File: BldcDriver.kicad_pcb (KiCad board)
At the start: 2 copper layers, 50 x 34 mm, 54 parts, among them J1 Motor Out, J2 DC Jack, J3 STM32_Debug_5pin, Q1 2SK4033, Q2 2SK4033, Q3 2SK4033, Q4 2SK4033, Q5 2SK4033, Q6 2SK4033, U1 IR2101, U2 IR2101, U3 IR2101, U4 NJM78L33SU3, U5 STM32F303K8Tx, X1 12MHz

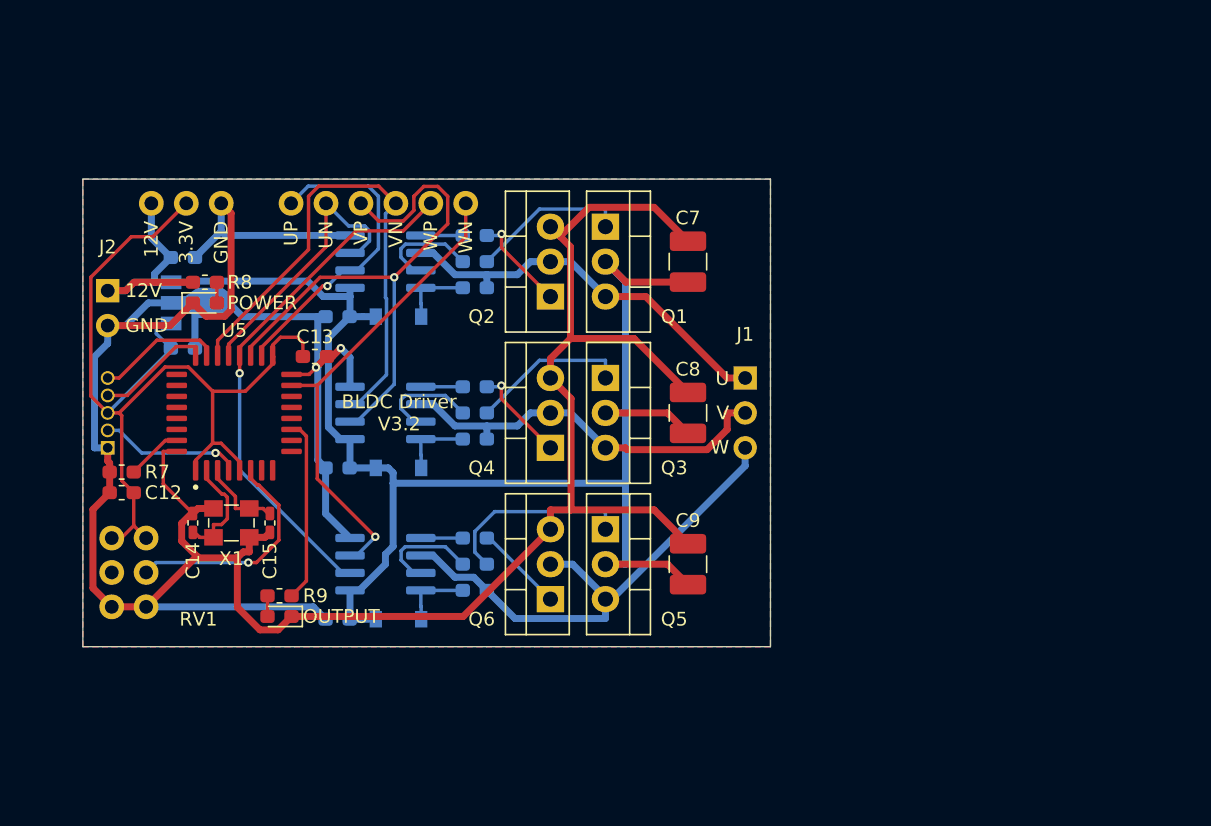
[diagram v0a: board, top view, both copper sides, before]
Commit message: 基板 V4.0
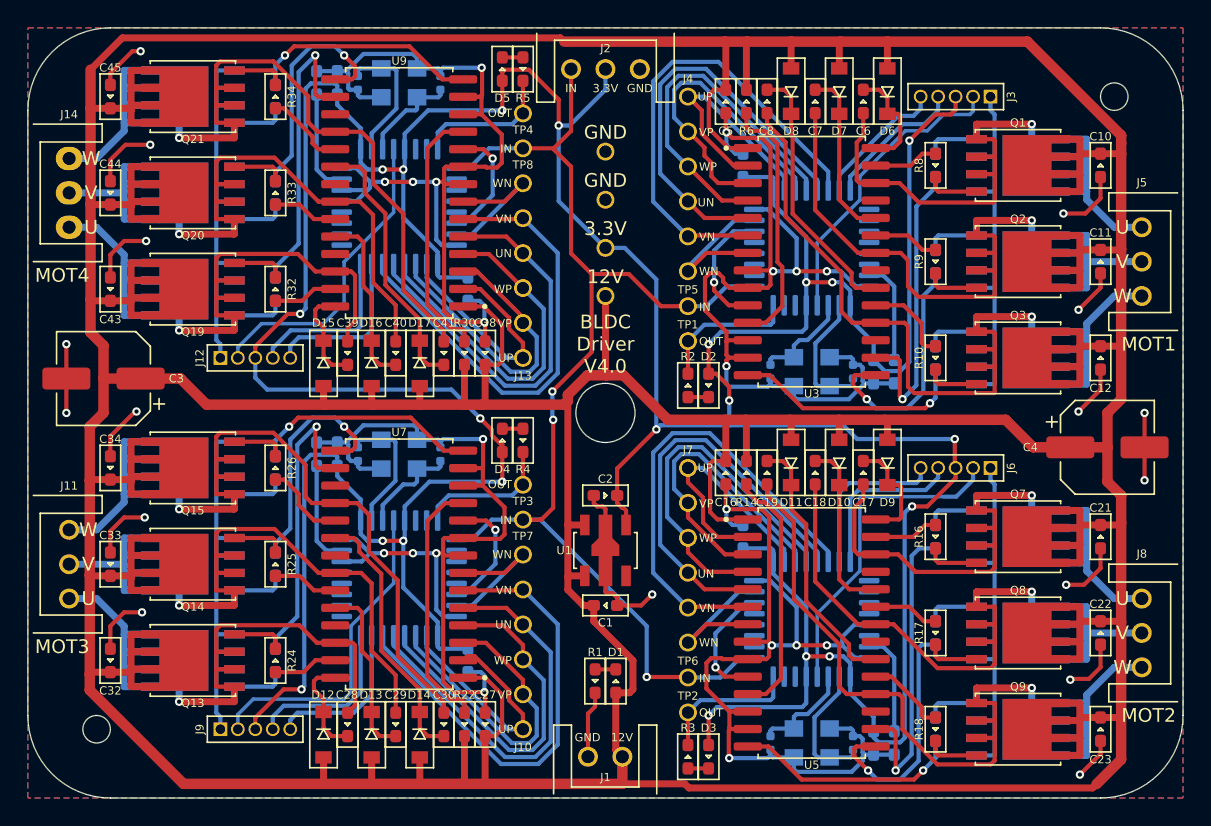
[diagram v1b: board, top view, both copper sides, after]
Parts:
- removed RV1: B10k, Potentiometer_THT:Potentiometer_Alps_RK097_Dual_Horizontal
- removed X1: 12MHz, BldcDriver:Crystal_SMD_3225-4Pin_3.2x2.5mm_HandSoldering
- added C16: 1uF, BldcDriver:1608Metric, F.Cu at (8.75, 4.35)
- added C17: 1uF, BldcDriver:1608Metric, F.Cu at (18.8, 4.35)
- added C18: 1uF, BldcDriver:1608Metric, F.Cu at (15.2, 4.35)
- added C19: 1uF, BldcDriver:1608Metric, F.Cu at (11.8, 4.35)
- added C20: 0.1uF, BldcDriver:1608Metric, B.Cu at (19.5, 24.0)
- added C21: 10uF, BldcDriver:1608Metric, F.Cu at (36.0, 9.00)
- added C22: 10uF, BldcDriver:1608Metric, F.Cu at (36.0, 16.0)
- added C23: 10uF, BldcDriver:1608Metric, F.Cu at (36.0, 23.0)
- added C24: 10pF, BldcDriver:1005Metric, B.Cu at (18.0, 24.0)
- added C25: 10pF, BldcDriver:1005Metric, B.Cu at (12.0, 24.0)
- added C26: 0.1uF, BldcDriver:1608Metric, B.Cu at (10.0, 9.00)
- added C27: 1uF, BldcDriver:1608Metric, F.Cu at (-8.75, 22.6)
- added C28: 1uF, BldcDriver:1608Metric, F.Cu at (-18.8, 22.6)
- added C29: 1uF, BldcDriver:1608Metric, F.Cu at (-15.2, 22.6)
- added C30: 1uF, BldcDriver:1608Metric, F.Cu at (-11.8, 22.6)
- added C31: 0.1uF, BldcDriver:1608Metric, B.Cu at (-19.5, 3.00)
- added C32: 10uF, BldcDriver:1608Metric, F.Cu at (-36.0, 18.0)
- added C33: 10uF, BldcDriver:1608Metric, F.Cu at (-36.0, 11.0)
- added C34: 10uF, BldcDriver:1608Metric, F.Cu at (-36.0, 4.00)
- added C35: 10pF, BldcDriver:1005Metric, B.Cu at (-18.0, 3.00)
- added C36: 10pF, BldcDriver:1005Metric, B.Cu at (-12.0, 3.00)
- added C37: 0.1uF, BldcDriver:1608Metric, B.Cu at (-10.0, 18.0)
- added C38: 1uF, BldcDriver:1608Metric, F.Cu at (-8.75, -4.35)
- added C39: 1uF, BldcDriver:1608Metric, F.Cu at (-18.8, -4.35)
- added C40: 1uF, BldcDriver:1608Metric, F.Cu at (-15.2, -4.35)
- added C41: 1uF, BldcDriver:1608Metric, F.Cu at (-11.8, -4.35)
- added C42: 0.1uF, BldcDriver:1608Metric, B.Cu at (-19.5, -24.0)
- added C43: 10uF, BldcDriver:1608Metric, F.Cu at (-36.0, -9.00)
- added C44: 10uF, BldcDriver:1608Metric, F.Cu at (-36.0, -16.0)
- added C45: 10uF, BldcDriver:1608Metric, F.Cu at (-36.0, -23.0)
- added C46: 10pF, BldcDriver:1005Metric, B.Cu at (-18.0, -24.0)
- added C47: 10pF, BldcDriver:1005Metric, B.Cu at (-12.0, -24.0)
- added C48: 0.1uF, BldcDriver:1608Metric, B.Cu at (-10.0, -9.00)
- added D10: 1N4148W, BldcDriver:D_SOD-123, F.Cu at (17.0, 3.60)
- added D11: 1N4148W, BldcDriver:D_SOD-123, F.Cu at (13.5, 3.60)
- added D12: 1N4148W, BldcDriver:D_SOD-123, F.Cu at (-20.5, 23.4)
- added D13: 1N4148W, BldcDriver:D_SOD-123, F.Cu at (-17.0, 23.4)
- added D14: 1N4148W, BldcDriver:D_SOD-123, F.Cu at (-13.5, 23.4)
- added D15: 1N4148W, BldcDriver:D_SOD-123, F.Cu at (-20.5, -3.60)
- added D16: 1N4148W, BldcDriver:D_SOD-123, F.Cu at (-17.0, -3.60)
- added D17: 1N4148W, BldcDriver:D_SOD-123, F.Cu at (-13.5, -3.60)
- added D6: 1N4148W, BldcDriver:D_SOD-123, F.Cu at (20.5, -23.4)
- added D7: 1N4148W, BldcDriver:D_SOD-123, F.Cu at (17.0, -23.4)
- added D8: 1N4148W, BldcDriver:D_SOD-123, F.Cu at (13.5, -23.4)
- added D9: 1N4148W, BldcDriver:D_SOD-123, F.Cu at (20.5, 3.60)
- added H1: MountingHole, BldcDriver:MountingHole_4.3mm_M4, F.Cu at (0.00, 0.00)
- added H2: MountingHole, BldcDriver:MountingHole_2mm, F.Cu at (37.0, -23.0)
- added H3: MountingHole, BldcDriver:MountingHole_2mm, F.Cu at (-37.0, 23.0)
- added J10: Conn_01x06, BldcDriver:Pin_1x06_P2.54mm, F.Cu at (-6.00, 23.0)
- added J11: MOTOR_OUT, BldcDriver:JST_XH_S3B-XH-A_1x03_P2.50mm_Horizontal, F.Cu at (-39.0, 8.50)
- added J12: STM32_Debug, BldcDriver:STM32_Debug_5pin, F.Cu at (-28.0, -4.00)
- added J13: Conn_01x06, BldcDriver:Pin_1x06_P2.54mm, F.Cu at (-6.00, -4.00)
- added J14: MOTOR_OUT, BldcDriver:JST_XH_S3B-XH-A_1x03_P2.50mm_Horizontal, F.Cu at (-39.0, -18.5)
- added J4: Conn_01x06, BldcDriver:Pin_1x06_P2.54mm, F.Cu at (6.00, -23.0)
- added J5: MOTOR_OUT, BldcDriver:JST_XH_S3B-XH-A_1x03_P2.50mm_Horizontal, F.Cu at (39.0, -8.50)
- added J6: STM32_Debug, BldcDriver:STM32_Debug_5pin, F.Cu at (28.0, 4.00)
- added J7: Conn_01x06, BldcDriver:Pin_1x06_P2.54mm, F.Cu at (6.00, 4.00)
- added J8: MOTOR_OUT, BldcDriver:JST_XH_S3B-XH-A_1x03_P2.50mm_Horizontal, F.Cu at (39.0, 18.5)
- added J9: STM32_Debug, BldcDriver:STM32_Debug_5pin, F.Cu at (-28.0, 23.0)
- added Q10: IRFH7545, BldcDriver:VSONP-8-1EP_5x6_P1.27mm, B.Cu at (30.0, 9.00)
- added Q11: IRFH7545, BldcDriver:VSONP-8-1EP_5x6_P1.27mm, B.Cu at (30.0, 16.0)
- added Q12: IRFH7545, BldcDriver:VSONP-8-1EP_5x6_P1.27mm, B.Cu at (30.0, 23.0)
- added Q13: IRFH7545, BldcDriver:VSONP-8-1EP_5x6_P1.27mm, F.Cu at (-30.0, 18.0)
- added Q14: IRFH7545, BldcDriver:VSONP-8-1EP_5x6_P1.27mm, F.Cu at (-30.0, 11.0)
- added Q15: IRFH7545, BldcDriver:VSONP-8-1EP_5x6_P1.27mm, F.Cu at (-30.0, 4.00)
- added Q16: IRFH7545, BldcDriver:VSONP-8-1EP_5x6_P1.27mm, B.Cu at (-30.0, 18.0)
- added Q17: IRFH7545, BldcDriver:VSONP-8-1EP_5x6_P1.27mm, B.Cu at (-30.0, 11.0)
- added Q18: IRFH7545, BldcDriver:VSONP-8-1EP_5x6_P1.27mm, B.Cu at (-30.0, 4.00)
- added Q19: IRFH7545, BldcDriver:VSONP-8-1EP_5x6_P1.27mm, F.Cu at (-30.0, -9.00)
- added Q20: IRFH7545, BldcDriver:VSONP-8-1EP_5x6_P1.27mm, F.Cu at (-30.0, -16.0)
- added Q21: IRFH7545, BldcDriver:VSONP-8-1EP_5x6_P1.27mm, F.Cu at (-30.0, -23.0)
- added Q22: IRFH7545, BldcDriver:VSONP-8-1EP_5x6_P1.27mm, B.Cu at (-30.0, -9.00)
- added Q23: IRFH7545, BldcDriver:VSONP-8-1EP_5x6_P1.27mm, B.Cu at (-30.0, -16.0)
- added Q24: IRFH7545, BldcDriver:VSONP-8-1EP_5x6_P1.27mm, B.Cu at (-30.0, -23.0)
- added Q7: IRFH7545, BldcDriver:VSONP-8-1EP_5x6_P1.27mm, F.Cu at (30.0, 9.00)
- added Q8: IRFH7545, BldcDriver:VSONP-8-1EP_5x6_P1.27mm, F.Cu at (30.0, 16.0)
- added Q9: IRFH7545, BldcDriver:VSONP-8-1EP_5x6_P1.27mm, F.Cu at (30.0, 23.0)
- added R10: 100, BldcDriver:1608Metric, F.Cu at (24.0, -4.00)
- added R11: 100, BldcDriver:1608Metric, B.Cu at (24.0, -18.0)
- added R12: 100, BldcDriver:1608Metric, B.Cu at (24.0, -11.0)
- added R13: 100, BldcDriver:1608Metric, B.Cu at (24.0, -4.00)
- added R14: 10k, BldcDriver:1608Metric, F.Cu at (10.2, 4.35)
- added R15: 10k, BldcDriver:1608Metric, B.Cu at (21.0, 24.0)
- added R16: 100, BldcDriver:1608Metric, F.Cu at (24.0, 9.00)
- added R17: 100, BldcDriver:1608Metric, F.Cu at (24.0, 16.0)
- added R18: 100, BldcDriver:1608Metric, F.Cu at (24.0, 23.0)
- added R19: 100, BldcDriver:1608Metric, B.Cu at (24.0, 9.00)
- added R20: 100, BldcDriver:1608Metric, B.Cu at (24.0, 16.0)
- added R21: 100, BldcDriver:1608Metric, B.Cu at (24.0, 23.0)
- added R22: 10k, BldcDriver:1608Metric, F.Cu at (-10.2, 22.6)
- added R23: 10k, BldcDriver:1608Metric, B.Cu at (-21.0, 3.00)
- added R24: 100, BldcDriver:1608Metric, F.Cu at (-24.0, 18.0)
- added R25: 100, BldcDriver:1608Metric, F.Cu at (-24.0, 11.0)
- added R26: 100, BldcDriver:1608Metric, F.Cu at (-24.0, 4.00)
- added R27: 100, BldcDriver:1608Metric, B.Cu at (-24.0, 18.0)
- added R28: 100, BldcDriver:1608Metric, B.Cu at (-24.0, 11.0)
- added R29: 100, BldcDriver:1608Metric, B.Cu at (-24.0, 4.00)
- added R30: 10k, BldcDriver:1608Metric, F.Cu at (-10.2, -4.35)
- added R31: 10k, BldcDriver:1608Metric, B.Cu at (-21.0, -24.0)
- added R32: 100, BldcDriver:1608Metric, F.Cu at (-24.0, -9.00)
- added R33: 100, BldcDriver:1608Metric, F.Cu at (-24.0, -16.0)
- added R34: 100, BldcDriver:1608Metric, F.Cu at (-24.0, -23.0)
- added R35: 100, BldcDriver:1608Metric, B.Cu at (-24.0, -9.00)
- added R36: 100, BldcDriver:1608Metric, B.Cu at (-24.0, -16.0)
- added R37: 100, BldcDriver:1608Metric, B.Cu at (-24.0, -23.0)
- added TP10: TestPoint, BldcDriver:TestPoint_THTPad_D1.3mm_Drill0.9mm, F.Cu at (0.00, -12.0)
- added TP11: TestPoint, BldcDriver:TestPoint_THTPad_D1.3mm_Drill0.9mm, F.Cu at (0.00, -15.5)
- added TP12: TestPoint, BldcDriver:TestPoint_THTPad_D1.3mm_Drill0.9mm, F.Cu at (0.00, -19.0)
- added U6: STM32F303K8Tx, BldcDriver:LQFP-32_7x7mm_P0.8mm_FusionPCB, B.Cu at (-15.0, 12.0)
- added U7: IR2136S, BldcDriver:SOIC-28W_7.5x17.9mm_P1.27mm, F.Cu at (-15.0, 11.0)
- added U8: STM32F303K8Tx, BldcDriver:LQFP-32_7x7mm_P0.8mm_FusionPCB, B.Cu at (-15.0, -15.0)
- added U9: IR2136S, BldcDriver:SOIC-28W_7.5x17.9mm_P1.27mm, F.Cu at (-15.0, -16.0)
- added Y1: 12MHz, BldcDriver:Crystal_SMD_3225-4Pin_3.2x2.5mm_HandSoldering, B.Cu at (15.0, -3.00)
- added Y2: 12MHz, BldcDriver:Crystal_SMD_3225-4Pin_3.2x2.5mm_HandSoldering, B.Cu at (15.0, 24.0)
- added Y3: 12MHz, BldcDriver:Crystal_SMD_3225-4Pin_3.2x2.5mm_HandSoldering, B.Cu at (-15.0, 3.00)
- added Y4: 12MHz, BldcDriver:Crystal_SMD_3225-4Pin_3.2x2.5mm_HandSoldering, B.Cu at (-15.0, -24.0)
- C1: value 10uF -> 0.33uF; footprint Capacitor_SMD:C_0603_1608Metric_Pad1.05x0.95mm_HandSolder -> BldcDriver:1608Metric; moved to F.Cu
- C10: value 0.39uF -> 10uF; footprint Capacitor_SMD:C_0603_1608Metric_Pad1.05x0.95mm_HandSolder -> BldcDriver:1608Metric; moved to F.Cu
- C11: value 0.1uF -> 10uF; footprint Capacitor_SMD:C_0603_1608Metric_Pad1.05x0.95mm_HandSolder -> BldcDriver:1608Metric; moved to F.Cu
- C12: value 0.1uF -> 10uF; footprint Capacitor_SMD:C_0603_1608Metric_Pad1.05x0.95mm_HandSolder -> BldcDriver:1608Metric
- C13: value 0.1uF -> 10pF; footprint Capacitor_SMD:C_0603_1608Metric_Pad1.05x0.95mm_HandSolder -> BldcDriver:1005Metric; moved to B.Cu
- C14: footprint BldcDriver:C_0402_1005Metric -> BldcDriver:1005Metric; moved to B.Cu
- C15: value 10pF -> 0.1uF; footprint BldcDriver:C_0402_1005Metric -> BldcDriver:1608Metric; moved to B.Cu
- C2: value 10uF -> 2.2uF; footprint Capacitor_SMD:C_0603_1608Metric_Pad1.05x0.95mm_HandSolder -> BldcDriver:1608Metric; moved to F.Cu
- C3, C4: value 10uF -> 100uF; footprint Capacitor_SMD:C_0603_1608Metric_Pad1.05x0.95mm_HandSolder -> BldcDriver:CP_Elec_6.3x7.7; moved to F.Cu
- C5, C6: value 10uF -> 1uF; footprint Capacitor_SMD:C_0603_1608Metric_Pad1.05x0.95mm_HandSolder -> BldcDriver:1608Metric; moved to F.Cu
- C7, C8: value 22uF -> 1uF; footprint Capacitor_SMD:C_1210_3225Metric_Pad1.42x2.65mm_HandSolder -> BldcDriver:1608Metric
- C9: value 22uF -> 0.1uF; footprint Capacitor_SMD:C_1210_3225Metric_Pad1.42x2.65mm_HandSolder -> BldcDriver:1608Metric; moved to B.Cu
- D1: value 1N4148W -> Power; footprint Diode_SMD:D_SOD-123 -> BldcDriver:1608Metric; moved to F.Cu
- D2: value 1N4148W -> OUT1; footprint Diode_SMD:D_SOD-123 -> BldcDriver:1608Metric; moved to F.Cu
- D3: value 1N4148W -> OUT2; footprint Diode_SMD:D_SOD-123 -> BldcDriver:1608Metric; moved to F.Cu
- D4: value Power -> OUT3; footprint LED_SMD:LED_0603_1608Metric_Pad1.05x0.95mm_HandSolder -> BldcDriver:1608Metric
- D5: value Output -> OUT4; footprint LED_SMD:LED_0603_1608Metric_Pad1.05x0.95mm_HandSolder -> BldcDriver:1608Metric
- J1: value Motor Out -> POWER; footprint Connector_PinSocket_2.54mm:PinSocket_1x03_P2.54mm_Vertical -> BldcDriver:JST_XH_S2B-XH-A_1x02_P2.50mm_Horizontal
- J2: value DC Jack -> CONTROL; footprint Connector_PinSocket_2.54mm:PinSocket_1x02_P2.54mm_Vertical -> BldcDriver:JST_XH_S3B-XH-A_1x03_P2.50mm_Horizontal
- J3: value STM32_Debug_5pin -> STM32_Debug; moved to F.Cu
- Q1, Q2, Q3: value 2SK4033 -> IRFH7545; footprint Package_TO_SOT_THT:TO-220-3_Vertical -> BldcDriver:VSONP-8-1EP_5x6_P1.27mm
- Q4, Q5, Q6: value 2SK4033 -> IRFH7545; footprint Package_TO_SOT_THT:TO-220-3_Vertical -> BldcDriver:VSONP-8-1EP_5x6_P1.27mm; moved to B.Cu
- R1, R2, R3, R4, R5: value 100 -> R; footprint Resistor_SMD:R_0603_1608Metric_Pad1.05x0.95mm_HandSolder -> BldcDriver:1608Metric; moved to F.Cu
- R6: value 100 -> 10k; footprint Resistor_SMD:R_0603_1608Metric_Pad1.05x0.95mm_HandSolder -> BldcDriver:1608Metric; moved to F.Cu
- R7: footprint Resistor_SMD:R_0603_1608Metric_Pad1.05x0.95mm_HandSolder -> BldcDriver:1608Metric; moved to B.Cu
- R8, R9: value R -> 100; footprint Resistor_SMD:R_0603_1608Metric_Pad1.05x0.95mm_HandSolder -> BldcDriver:1608Metric
- TP1: value +12V -> TestPoint; footprint BldcDriver:TestPoint_THTPad_D2.0mm_Drill1.0mm -> BldcDriver:TestPoint_THTPad_D1.3mm_Drill0.9mm
- TP2: value GND -> TestPoint; footprint BldcDriver:TestPoint_THTPad_D2.0mm_Drill1.0mm -> BldcDriver:TestPoint_THTPad_D1.3mm_Drill0.9mm
- TP3: value 3.3V -> TestPoint; footprint BldcDriver:TestPoint_THTPad_D2.0mm_Drill1.0mm -> BldcDriver:TestPoint_THTPad_D1.3mm_Drill0.9mm
- TP4: value UP -> TestPoint; footprint BldcDriver:TestPoint_THTPad_D2.0mm_Drill1.0mm -> BldcDriver:TestPoint_THTPad_D1.3mm_Drill0.9mm
- TP5: value UN -> TestPoint; footprint BldcDriver:TestPoint_THTPad_D2.0mm_Drill1.0mm -> BldcDriver:TestPoint_THTPad_D1.3mm_Drill0.9mm
- TP6: value VP -> TestPoint; footprint BldcDriver:TestPoint_THTPad_D2.0mm_Drill1.0mm -> BldcDriver:TestPoint_THTPad_D1.3mm_Drill0.9mm
- TP7: value VN -> TestPoint; footprint BldcDriver:TestPoint_THTPad_D2.0mm_Drill1.0mm -> BldcDriver:TestPoint_THTPad_D1.3mm_Drill0.9mm
- TP8: value WP -> TestPoint; footprint BldcDriver:TestPoint_THTPad_D2.0mm_Drill1.0mm -> BldcDriver:TestPoint_THTPad_D1.3mm_Drill0.9mm
- TP9: value WN -> TestPoint; footprint BldcDriver:TestPoint_THTPad_D2.0mm_Drill1.0mm -> BldcDriver:TestPoint_THTPad_D1.3mm_Drill0.9mm
- U1: value IR2101 -> NJM2884U1; footprint BldcDriver:SOIC-8_3.9x4.9mm_P1.27mm -> BldcDriver:SOT-89-5; moved to F.Cu
- U2: value IR2101 -> STM32F303K8Tx; footprint BldcDriver:SOIC-8_3.9x4.9mm_P1.27mm -> BldcDriver:LQFP-32_7x7mm_P0.8mm_FusionPCB
- U3: value IR2101 -> IR2136S; footprint BldcDriver:SOIC-8_3.9x4.9mm_P1.27mm -> BldcDriver:SOIC-28W_7.5x17.9mm_P1.27mm; moved to F.Cu
- U4: value NJM78L33SU3 -> STM32F303K8Tx; footprint Package_TO_SOT_SMD:SOT-89-3 -> BldcDriver:LQFP-32_7x7mm_P0.8mm_FusionPCB
- U5: value STM32F303K8Tx -> IR2136S; footprint BldcDriver:LQFP-32_7x7mm_P0.8mm_FusionPCB -> BldcDriver:SOIC-28W_7.5x17.9mm_P1.27mm
- moved C12 71.8 mm to (36.0, -4.00), turned to 270 degrees
- moved J3 69.1 mm to (28.0, -23.0), turned to 270 degrees
- moved C10 67.1 mm to (36.0, -18.0), turned to 270 degrees
- moved C11 67.0 mm to (36.0, -11.0), turned to 270 degrees
- moved R7 56.6 mm to (21.0, -3.00), turned to 270 degrees
- moved R8 53.8 mm to (24.0, -18.0), turned to 90 degrees
- moved R9 53.5 mm to (24.0, -11.0), turned to 90 degrees
- moved U4 50.6 mm to (15.0, 15.0), turned to 90 degrees
- moved TP2 50.2 mm to (6.00, 21.8)
- moved C4 47.4 mm to (36.5, 2.50)
- moved C6 45.4 mm to (18.8, -22.6), turned to 270 degrees
- moved C15 45.3 mm to (19.5, -3.00)
- moved U5 44.9 mm to (15.0, 16.0), turned to 0 degrees
- moved C14 43.4 mm to (12.0, -3.00), turned to 270 degrees
- moved D5 43.0 mm to (-7.50, -25.0), turned to 270 degrees
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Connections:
- C11 pad 1: +3V3 -> +12V
- C12 pad 1: +3V3 -> +12V
- C13 pad 1: +3V3 -> GND
- C13 pad 2: GND -> Net-(C13-Pad2)
- C14 pad 1: OSC_I -> Net-(C14-Pad1)
- C15 pad 1: OSC_O -> +3V3
- C2 pad 1: +12V -> +3V3
- C4 pad 1: Net-(C4-Pad1) -> +12V
- C4 pad 2: /U -> GND
- C5 pad 1: Net-(C5-Pad1) -> +12V
- C5 pad 2: /V -> GND
- C6 pad 2: /W -> /U1
- C7 pad 1: +12V -> Net-(C7-Pad1)
- C7 pad 2: GND -> /V1
- C8 pad 1: +12V -> Net-(C8-Pad1)
- C8 pad 2: GND -> /W1
- C9 pad 1: +12V -> +3V3
- D1 pad 1: Net-(C4-Pad1) -> Net-(D1-Pad1)
- D2 pad 1: Net-(C5-Pad1) -> Net-(D2-Pad1)
- D2 pad 2: +12V -> +3V3
- D3 pad 1: Net-(C6-Pad1) -> Net-(D3-Pad1)
- D3 pad 2: +12V -> +3V3
- D4 pad 1: GND -> Net-(D4-Pad1)
- D4 pad 2: Net-(D4-Pad2) -> +3V3
- D5 pad 1: GND -> Net-(D5-Pad1)
- D5 pad 2: Net-(D5-Pad2) -> +3V3
- J1 pad 1: /U -> +12V
- J1 pad 2: /V -> GND
- J2 pad 1: +12V -> IN1
- J2 pad 2: GND -> +3V3
- J3 pad 2: NRST -> Net-(J3-Pad2)
- J3 pad 4: SWCLK -> Net-(J3-Pad4)
- J3 pad 5: SWDIO -> Net-(J3-Pad5)
- Q1 pad 1: Net-(Q1-Pad1) -> /U1
- Q1 pad 2: +12V -> Net-(Q1-Pad2)
- Q1 pad 3: /U -> +12V
- Q2 pad 1: Net-(Q2-Pad1) -> /V1
- Q2 pad 2: /U -> Net-(Q2-Pad2)
- Q2 pad 3: GND -> +12V
- Q3 pad 1: Net-(Q3-Pad1) -> /W1
- Q3 pad 2: +12V -> Net-(Q3-Pad2)
- Q3 pad 3: /V -> +12V
- Q4 pad 1: Net-(Q4-Pad1) -> GND
- Q4 pad 2: /V -> Net-(Q4-Pad2)
- Q4 pad 3: GND -> /U1
- Q5 pad 1: Net-(Q5-Pad1) -> GND
- Q5 pad 2: +12V -> Net-(Q5-Pad2)
- Q5 pad 3: /W -> /V1
- Q6 pad 1: Net-(Q6-Pad1) -> GND
- Q6 pad 2: /W -> Net-(Q6-Pad2)
- Q6 pad 3: GND -> /W1
- R1 pad 1: Net-(Q1-Pad1) -> GND
- R1 pad 2: Net-(R1-Pad2) -> Net-(D1-Pad1)
- R2 pad 1: Net-(Q2-Pad1) -> OUT1
- R2 pad 2: Net-(R2-Pad2) -> Net-(D2-Pad1)
- R3 pad 1: Net-(Q3-Pad1) -> OUT2
- R3 pad 2: Net-(R3-Pad2) -> Net-(D3-Pad1)
- R4 pad 1: Net-(Q4-Pad1) -> OUT3
- R4 pad 2: Net-(R4-Pad2) -> Net-(D4-Pad1)
- R5 pad 1: Net-(Q5-Pad1) -> OUT4
- R5 pad 2: Net-(R5-Pad2) -> Net-(D5-Pad1)
- R6 pad 1: Net-(Q6-Pad1) -> +12V
- R8 pad 1: Net-(D4-Pad2) -> Net-(Q1-Pad2)
- R8 pad 2: +12V -> Net-(R8-Pad2)
- R9 pad 1: Net-(D5-Pad2) -> Net-(Q2-Pad2)
- R9 pad 2: LED -> Net-(R9-Pad2)
- TP1 pad 1: +12V -> OUT1
- TP2 pad 1: GND -> OUT2
- TP3 pad 1: +3V3 -> OUT3
- TP4 pad 1: UP -> OUT4
- TP5 pad 1: UN -> IN1
- TP6 pad 1: VP -> IN1
- TP7 pad 1: VN -> IN1
- TP8 pad 1: WP -> IN1
- TP9 pad 1: WN -> +12V
- U1 pad 2: UP -> GND
- U1 pad 3: UN -> Net-(U1-Pad3)
- U1 pad 4: GND -> +3V3
- U1 pad 5: Net-(R2-Pad2) -> +12V
- U2 pad 1: +12V -> +3V3
- U2 pad 2: VP -> Net-(C13-Pad2)
- U2 pad 3: VN -> Net-(C14-Pad1)
- U2 pad 4: GND -> Net-(J3-Pad2)
- U2 pad 5: Net-(R4-Pad2) -> +3V3
- U2 pad 6: /V -> Net-(U2-Pad6)
- U2 pad 7: Net-(R3-Pad2) -> Net-(U2-Pad7)
- U2 pad 8: Net-(C5-Pad1) -> OUT1
- U3 pad 2: WP -> /UP1
- U3 pad 3: WN -> /VP1
- U3 pad 4: GND -> /WP1
- U3 pad 5: Net-(R6-Pad2) -> /UN1
- U3 pad 6: /W -> /VN1
- U3 pad 7: Net-(R5-Pad2) -> /WN1
- U3 pad 8: Net-(C6-Pad1) -> GND
- U4 pad 2: GND -> Net-(C24-Pad2)
- U4 pad 3: +12V -> Net-(C25-Pad1)
- U5 pad 1: +3V3 -> +12V
- U5 pad 10: (no net) -> Net-(U4-Pad14)
- U5 pad 11: LED -> Net-(R14-Pad2)
- U5 pad 12: (no net) -> GND
- U5 pad 13: (no net) -> GND
- U5 pad 14: (no net) -> Net-(R21-Pad2)
- U5 pad 15: WN -> Net-(R20-Pad2)
- U5 pad 16: GND -> Net-(R19-Pad2)
- U5 pad 17: +3V3 -> Net-(U5-Pad17)
- U5 pad 18: UP -> /W2
- U5 pad 19: VP -> Net-(R18-Pad2)
- U5 pad 2: OSC_I -> /UP2
- U5 pad 20: WP -> Net-(C19-Pad1)
- U5 pad 21: UN -> Net-(U5-Pad21)
- U5 pad 22: VN -> /V2
- U5 pad 23: SWDIO -> Net-(R17-Pad2)
- U5 pad 24: SWCLK -> Net-(C18-Pad1)
- U5 pad 25: (no net) -> Net-(U5-Pad25)
- U5 pad 26: (no net) -> /U2
- U5 pad 27: (no net) -> Net-(R16-Pad2)
- U5 pad 28: (no net) -> Net-(C17-Pad1)
- U5 pad 3: OSC_O -> /VP2
- U5 pad 4: NRST -> /WP2
- U5 pad 5: +3V3 -> /UN2
- U5 pad 6: ADC -> /VN2
- U5 pad 7: (no net) -> /WN2
- U5 pad 8: (no net) -> GND
- U5 pad 9: (no net) -> GND
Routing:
- net +12V: track 128.1 -> 625.7 mm
- net +3V3: track 70.7 -> 329.5 mm, vias 0 -> 21
- net GND: track 226.5 -> 484.3 mm, vias 2 -> 37
- net IN1: track 0.00 -> 88.1 mm, vias 0 -> 3
- net /W1: track 0.00 -> 69.0 mm, vias 0 -> 1
- net /W2: track 0.00 -> 68.0 mm, vias 0 -> 1
- net /W3: track 0.00 -> 67.7 mm, vias 0 -> 1
- net /W4: track 0.00 -> 67.7 mm, vias 0 -> 1
- net /V1: track 0.00 -> 58.6 mm, vias 0 -> 1
- net /V3: track 0.00 -> 57.8 mm, vias 0 -> 1
- net /V4: track 0.00 -> 57.8 mm, vias 0 -> 1
- net /V2: track 0.00 -> 57.5 mm, vias 0 -> 1
- net /U1: track 0.00 -> 52.1 mm, vias 0 -> 1
- net /U2: track 0.00 -> 52.0 mm, vias 0 -> 1
- net /U3: track 0.00 -> 52.0 mm, vias 0 -> 1
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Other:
- board size 50 x 34 mm -> 84 x 56 mm
- net class Default: trace_width 0.254 -> 0.3048
- net class Power removed
- rule pad_to_mask_clearance: 0.051 -> 0
- board text added: "BLDC Driver V4.0"
- board text added: "IN"
- board text added: "MOT1"
- board text added: "MOT2"
- board text added: "MOT3"
- board text added: "MOT4"
- board text added: "OUT"
- board text removed: "BLDC Driver V3.2"
- board text removed: "OUTPUT"
- board text removed: "POWER"
